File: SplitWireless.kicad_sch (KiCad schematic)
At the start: 57 parts, among them J1 OLED_128x32, SW1 Switch, SW2 Push_Button, U2 Nice_Nano_V2

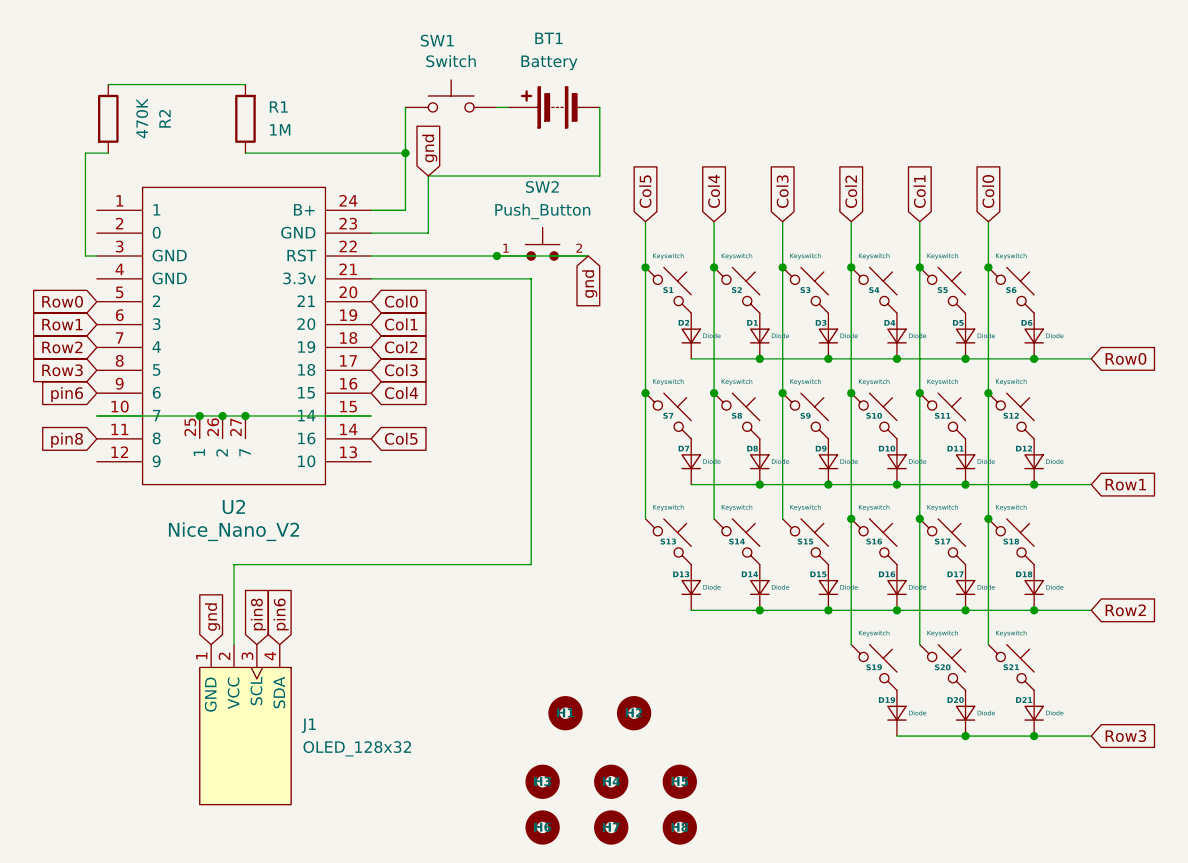
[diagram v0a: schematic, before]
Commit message: added some stuff
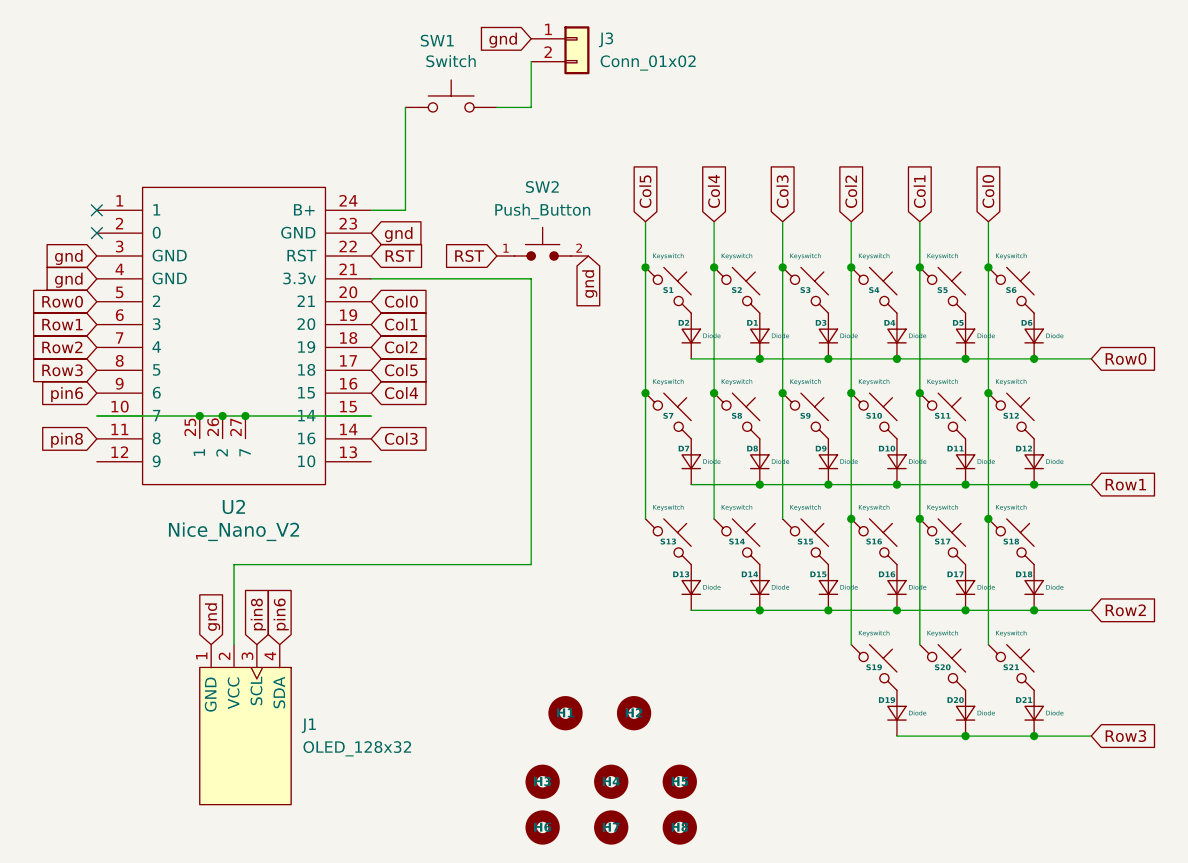
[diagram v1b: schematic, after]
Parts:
- removed BT1: Battery, ScottoKeebs_Scotto:Battery, symbol Device:Battery
- removed R1: 1M, ScottoKeebs_Components:Resistor_0805, symbol ScottoKeebs:Placeholder_Resistor
- removed R2: 470K, ScottoKeebs_Components:Resistor_0805, symbol ScottoKeebs:Placeholder_Resistor
- added J3: Conn_01x02, ScottoKeebs_Components:Connector_1x02_JST-PH, symbol PCM_4ms_Connector:Conn_01x02
- SW2: footprint Button_Switch_SMD:SW_SPST_TL3342 -> Button_Switch_SMD:Panasonic_EVQPUJ_EVQPUA
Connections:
- net Col3: now also U2.14 (16); no longer U2.17 (18)
- net Col5: now also U2.17 (18); no longer U2.14 (16)
- net gnd: now also U2.3 (GND), U2.4 (GND), J3.1 (Pin_1); no longer SW2.1, U2.22 (RST)
- net at SW1.2: now also J3.2 (Pin_2)
- new net RST: SW2.1, U2.22 (RST)
- no-connect marks 0 -> 2

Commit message: removed choc and some shit
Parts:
- S1, S10, S11, S12, S13, S14, S15, S16, S17, S18, S19, S2, S20, S21, S3, S4, S5, S6, S7, S8, S9: footprint ScottoKeebs_Scotto:Choc_Hotswap_1.00u -> ScottoKeebs_Scotto:MX_Hotswap_1.00u
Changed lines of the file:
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@@
 			)
 		)
-		(property "Footprint" "ScottoKeebs_Scotto:Choc_Hotswap_1.00u"
+		(property "Footprint" "ScottoKeebs_Scotto:MX_Hotswap_1.00u"
 			(at 158.75 59.69 0)
 			(effects
@@
 			)
 		)
-		(property "Footprint" "ScottoKeebs_Scotto:Choc_Hotswap_1.00u"
+		(property "Footprint" "ScottoKeebs_Scotto:MX_Hotswap_1.00u"
 			(at 173.99 73.66 0)
 			(effects
@@
 			)
 		)
-		(property "Footprint" "ScottoKeebs_Scotto:Choc_Hotswap_1.00u"
+		(property "Footprint" "ScottoKeebs_Scotto:MX_Hotswap_1.00u"
 			(at 135.89 87.63 0)
 			(effects
@@
 			)
 		)
-		(property "Footprint" "ScottoKeebs_Scotto:Choc_Hotswap_1.00u"
+		(property "Footprint" "ScottoKeebs_Scotto:MX_Hotswap_1.00u"
 			(at 158.75 101.6 0)
 			(effects
@@
 			)
 		)
-		(property "Footprint" "ScottoKeebs_Scotto:Choc_Hotswap_1.00u"
+		(property "Footprint" "ScottoKeebs_Scotto:MX_Hotswap_1.00u"
 			(at 166.37 87.63 0)
 			(effects
@@
 			)
 		)
-		(property "Footprint" "ScottoKeebs_Scotto:Choc_Hotswap_1.00u"
+		(property "Footprint" "ScottoKeebs_Scotto:MX_Hotswap_1.00u"
 			(at 143.51 87.63 0)
 			(effects
@@
 			)
 		)
-		(property "Footprint" "ScottoKeebs_Scotto:Choc_Hotswap_1.00u"
+		(property "Footprint" "ScottoKeebs_Scotto:MX_Hotswap_1.00u"
 			(at 166.37 59.69 0)
 			(effects
@@
 			)
 		)
-		(property "Footprint" "ScottoKeebs_Scotto:Choc_Hotswap_1.00u"
+		(property "Footprint" "ScottoKeebs_Scotto:MX_Hotswap_1.00u"
 			(at 151.13 59.69 0)
 			(effects
@@
 			)
 		)
-		(property "Footprint" "ScottoKeebs_Scotto:Choc_Hotswap_1.00u"
+		(property "Footprint" "ScottoKeebs_Scotto:MX_Hotswap_1.00u"
 			(at 173.99 101.6 0)
 			(effects
@@
 			)
 		)
-		(property "Footprint" "ScottoKeebs_Scotto:Choc_Hotswap_1.00u"
+		(property "Footprint" "ScottoKeebs_Scotto:MX_Hotswap_1.00u"
 			(at 158.75 87.63 0)
 			(effects
@@
 			)
 		)
-		(property "Footprint" "ScottoKeebs_Scotto:Choc_Hotswap_1.00u"
+		(property "Footprint" "ScottoKeebs_Scotto:MX_Hotswap_1.00u"
 			(at 135.89 59.69 0)
 			(effects
@@
 			)
 		)
-		(property "Footprint" "ScottoKeebs_Scotto:Choc_Hotswap_1.00u"
+		(property "Footprint" "ScottoKeebs_Scotto:MX_Hotswap_1.00u"
 			(at 151.13 73.66 0)
 			(effects
@@
 			)
 		)
-		(property "Footprint" "ScottoKeebs_Scotto:Choc_Hotswap_1.00u"
+		(property "Footprint" "ScottoKeebs_Scotto:MX_Hotswap_1.00u"
 			(at 158.75 73.66 0)
 			(effects
@@
 			)
 		)
-		(property "Footprint" "ScottoKeebs_Scotto:Choc_Hotswap_1.00u"
+		(property "Footprint" "ScottoKeebs_Scotto:MX_Hotswap_1.00u"
 			(at 166.37 73.66 0)
 			(effects
@@
 			)
 		)
-		(property "Footprint" "ScottoKeebs_Scotto:Choc_Hotswap_1.00u"
+		(property "Footprint" "ScottoKeebs_Scotto:MX_Hotswap_1.00u"
 			(at 135.89 73.66 0)
 			(effects
@@
 			)
 		)
-		(property "Footprint" "ScottoKeebs_Scotto:Choc_Hotswap_1.00u"
+		(property "Footprint" "ScottoKeebs_Scotto:MX_Hotswap_1.00u"
 			(at 173.99 87.63 0)
 			(effects
@@
 			)
 		)
-		(property "Footprint" "ScottoKeebs_Scotto:Choc_Hotswap_1.00u"
+		(property "Footprint" "ScottoKeebs_Scotto:MX_Hotswap_1.00u"
 			(at 151.13 87.63 0)
 			(effects
@@
 			)
 		)
-		(property "Footprint" "ScottoKeebs_Scotto:Choc_Hotswap_1.00u"
+		(property "Footprint" "ScottoKeebs_Scotto:MX_Hotswap_1.00u"
 			(at 143.51 73.66 0)
 			(effects
@@
 			)
 		)
-		(property "Footprint" "ScottoKeebs_Scotto:Choc_Hotswap_1.00u"
+		(property "Footprint" "ScottoKeebs_Scotto:MX_Hotswap_1.00u"
 			(at 173.99 59.69 0)
 			(effects
@@
 			)
 		)
-		(property "Footprint" "ScottoKeebs_Scotto:Choc_Hotswap_1.00u"
+		(property "Footprint" "ScottoKeebs_Scotto:MX_Hotswap_1.00u"
 			(at 143.51 59.69 0)
 			(effects
@@
 			)
 		)
-		(property "Footprint" "ScottoKeebs_Scotto:Choc_Hotswap_1.00u"
+		(property "Footprint" "ScottoKeebs_Scotto:MX_Hotswap_1.00u"
 			(at 166.37 101.6 0)
 			(effects

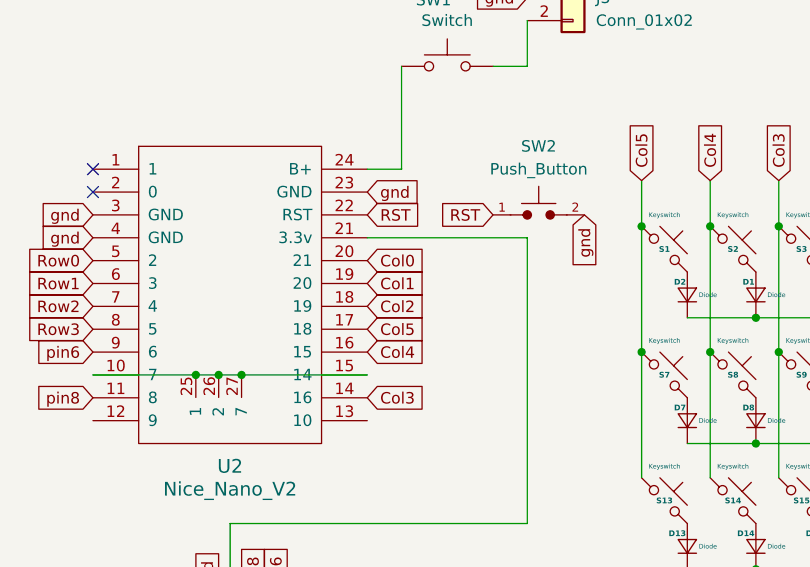
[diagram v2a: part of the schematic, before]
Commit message: workin
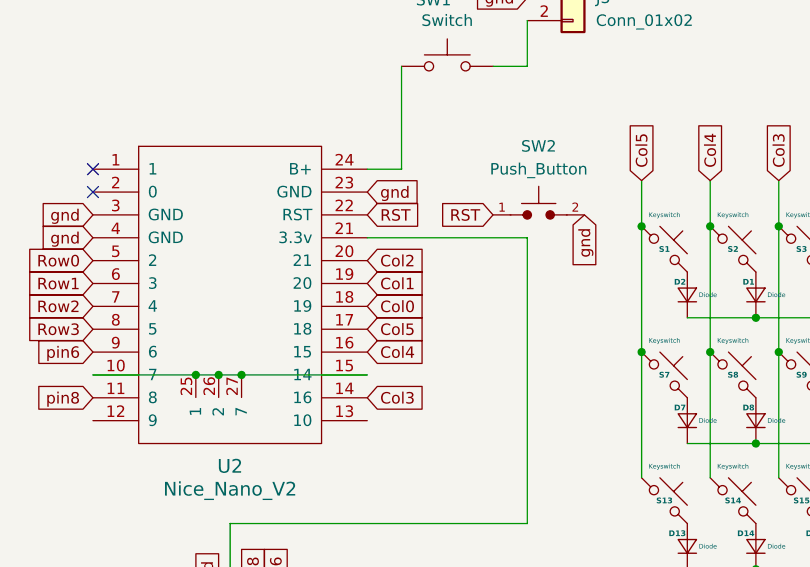
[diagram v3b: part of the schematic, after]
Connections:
- net Col0: now also U2.18 (19); no longer U2.20 (21)
- net Col2: now also U2.20 (21); no longer U2.18 (19)
